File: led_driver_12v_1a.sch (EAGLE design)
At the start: 53 parts, among them Q1 BSZ0902NSI, Q2 BSZ0902NSI, Q3 BSZ0902NSI, Q4 BSZ0902NSI, Q5 BSZ0902NSI, Q6 SSM3K2615R

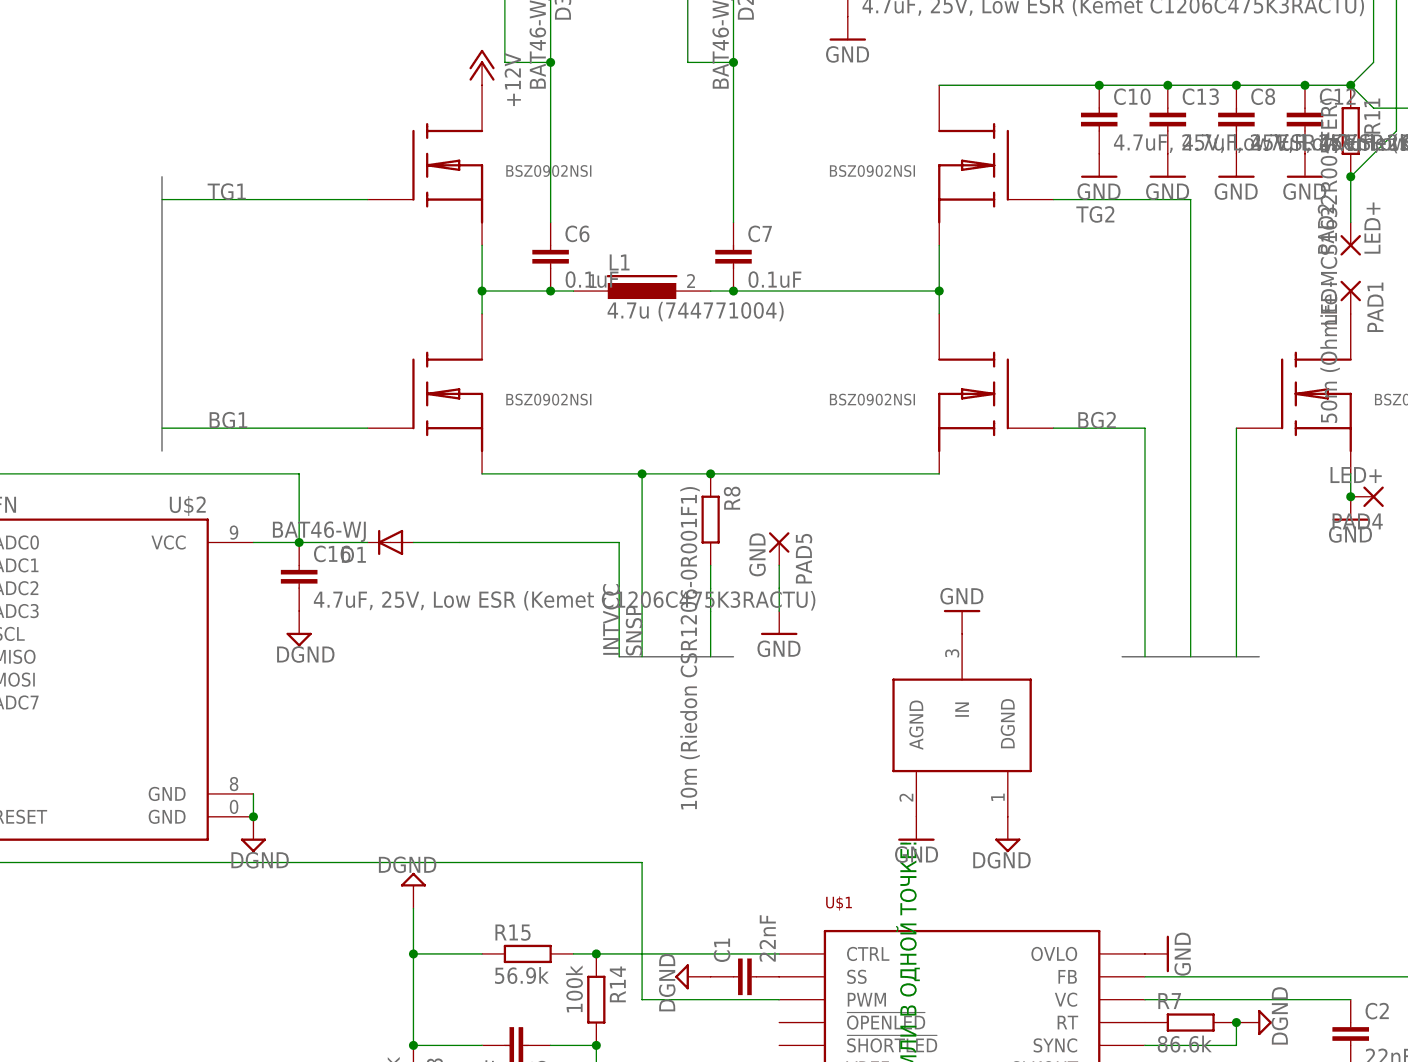
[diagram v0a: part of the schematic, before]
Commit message: routing complete. main tasks to do: add polys, optimize routes width, add some extra vias, make gerbers
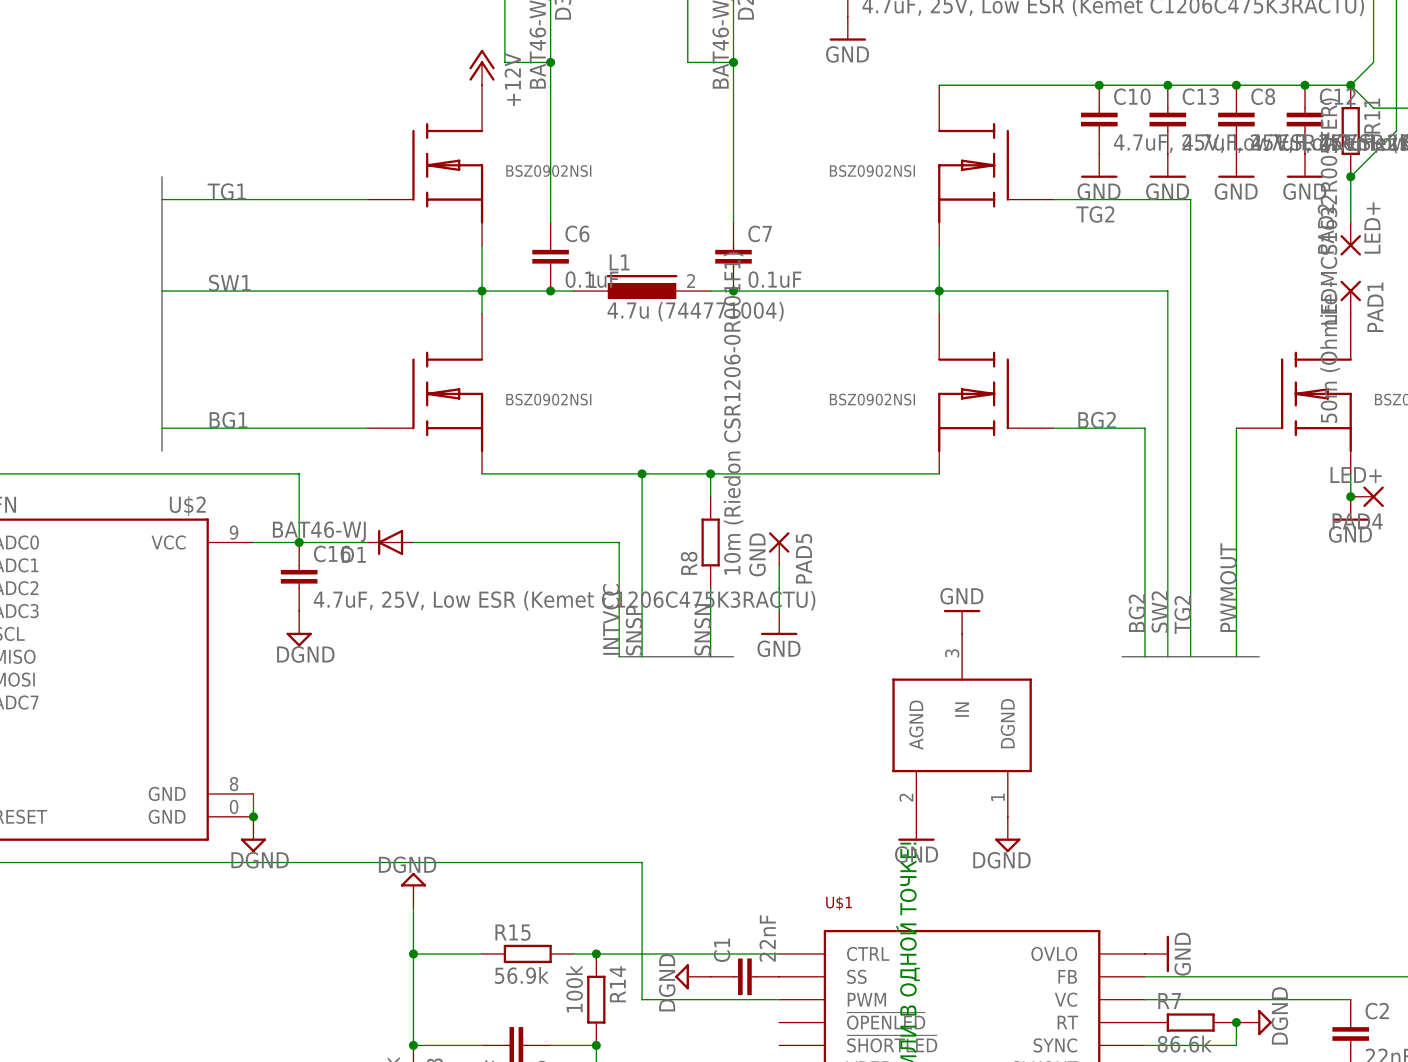
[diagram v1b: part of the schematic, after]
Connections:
- removed net N$10: C7.2, L1.2, Q3.D, Q4.S
- removed net N$8: C6.2, L1.1, Q1.S, Q2.D
- net SNSN: now also R8.1; no longer R8.2
- net SNSP: now also R8.2; no longer R8.1
- net SW1: now also C6.2, L1.1, Q1.S, Q2.D
- net SW2: now also C7.2, L1.2, Q3.D, Q4.S
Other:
- moved on the sheet: R8
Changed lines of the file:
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@@
 <clearance class="0" value="0.1524"/>
 </class>
-<class number="1" name="HI_PWR" width="0.3" drill="0.5">
+<class number="1" name="HI_PWR" width="0.3" drill="0.4">
 <clearance class="1" value="0.15"/>
 </class>
@@
 <instance part="Q3" gate="G$1" x="5.08" y="50.8" rot="MR0"/>
 <instance part="Q5" gate="G$1" x="45.72" y="50.8"/>
-<instance part="R8" gate="G$1" x="-22.86" y="38.1" rot="R270"/>
+<instance part="R8" gate="G$1" x="-22.86" y="35.56" rot="R90"/>
 <instance part="R11" gate="G$1" x="48.26" y="81.28" rot="R270"/>
 <instance part="D2" gate="G$1" x="-20.32" y="99.06" rot="R270"/>
@@
 <wire x1="25.4" y1="48.26" x2="25.4" y2="22.86" width="0.1524" layer="91"/>
 <label x="17.78" y="48.26" size="1.778" layer="95"/>
+<label x="25.4" y="25.4" size="1.778" layer="95" rot="R90"/>
 </segment>
 </net>
@@
 </segment>
 </net>
-<net name="SW2" class="0">
+<net name="SW2" class="1">
 <segment>
 <pinref part="U$1" gate="G$1" pin="SW2"/>
@@
 <label x="27.94" y="-53.34" size="1.778" layer="95"/>
 </segment>
-</net>
-<net name="SW1" class="0">
+<segment>
+<pinref part="L1" gate="G$1" pin="2"/>
+<pinref part="C7" gate="G$1" pin="2"/>
+<wire x1="-22.86" y1="63.5" x2="-20.32" y2="63.5" width="0.1524" layer="91"/>
+<pinref part="Q4" gate="G$1" pin="S"/>
+<wire x1="-20.32" y1="63.5" x2="2.54" y2="63.5" width="0.1524" layer="91"/>
+<wire x1="2.54" y1="63.5" x2="2.54" y2="68.58" width="0.1524" layer="91"/>
+<junction x="-20.32" y="63.5"/>
+<pinref part="Q3" gate="G$1" pin="D"/>
+<wire x1="2.54" y1="63.5" x2="2.54" y2="60.96" width="0.1524" layer="91"/>
+<junction x="2.54" y="63.5"/>
+<wire x1="27.94" y1="22.86" x2="27.94" y2="63.5" width="0.1524" layer="91"/>
+<wire x1="27.94" y1="63.5" x2="2.54" y2="63.5" width="0.1524" layer="91"/>
+<label x="27.94" y="25.4" size="1.778" layer="95" rot="R90"/>
+</segment>
+</net>
+<net name="SW1" class="1">
 <segment>
 <pinref part="U$1" gate="G$1" pin="SW1"/>
 <wire x1="-15.24" y1="-48.26" x2="-25.4" y2="-48.26" width="0.1524" layer="91"/>
 <label x="-22.86" y="-48.26" size="1.778" layer="95"/>
+</segment>
+<segment>
+<pinref part="Q1" gate="G$1" pin="S"/>
+<pinref part="Q2" gate="G$1" pin="D"/>
+<wire x1="-48.26" y1="68.58" x2="-48.26" y2="63.5" width="0.1524" layer="91"/>
+<pinref part="L1" gate="G$1" pin="1"/>
+<wire x1="-48.26" y1="63.5" x2="-48.26" y2="60.96" width="0.1524" layer="91"/>
+<wire x1="-38.1" y1="63.5" x2="-40.64" y2="63.5" width="0.1524" layer="91"/>
+<junction x="-48.26" y="63.5"/>
+<pinref part="C6" gate="G$1" pin="2"/>
+<wire x1="-40.64" y1="63.5" x2="-48.26" y2="63.5" width="0.1524" layer="91"/>
+<junction x="-40.64" y="63.5"/>
+<wire x1="-83.82" y1="63.5" x2="-48.26" y2="63.5" width="0.1524" layer="91"/>
+<label x="-78.74" y="63.5" size="1.778" layer="95"/>
 </segment>
 </net>
@@
 <wire x1="30.48" y1="73.66" x2="30.48" y2="22.86" width="0.1524" layer="91"/>
 <label x="17.78" y="71.12" size="1.778" layer="95"/>
+<label x="30.48" y="25.4" size="1.778" layer="95" rot="R90"/>
 </segment>
 </net>
@@
 </segment>
 </net>
-<net name="N$8" class="1">
-<segment>
-<pinref part="Q1" gate="G$1" pin="S"/>
-<pinref part="Q2" gate="G$1" pin="D"/>
-<wire x1="-48.26" y1="68.58" x2="-48.26" y2="63.5" width="0.1524" layer="91"/>
-<pinref part="L1" gate="G$1" pin="1"/>
-<wire x1="-48.26" y1="63.5" x2="-48.26" y2="60.96" width="0.1524" layer="91"/>
-<wire x1="-38.1" y1="63.5" x2="-40.64" y2="63.5" width="0.1524" layer="91"/>
-<junction x="-48.26" y="63.5"/>
-<pinref part="C6" gate="G$1" pin="2"/>
-<wire x1="-40.64" y1="63.5" x2="-48.26" y2="63.5" width="0.1524" layer="91"/>
-<junction x="-40.64" y="63.5"/>
-</segment>
-</net>
-<net name="N$10" class="1">
-<segment>
-<pinref part="L1" gate="G$1" pin="2"/>
-<pinref part="C7" gate="G$1" pin="2"/>
-<wire x1="-22.86" y1="63.5" x2="-20.32" y2="63.5" width="0.1524" layer="91"/>
-<pinref part="Q4" gate="G$1" pin="S"/>
-<wire x1="-20.32" y1="63.5" x2="2.54" y2="63.5" width="0.1524" layer="91"/>
-<wire x1="2.54" y1="63.5" x2="2.54" y2="68.58" width="0.1524" layer="91"/>
-<junction x="-20.32" y="63.5"/>
-<pinref part="Q3" gate="G$1" pin="D"/>
-<wire x1="2.54" y1="63.5" x2="2.54" y2="60.96" width="0.1524" layer="91"/>
-<junction x="2.54" y="63.5"/>
-</segment>
-</net>
 <net name="PWMOUT" class="1">
 <segment>
@@
 <pinref part="Q5" gate="G$1" pin="G"/>
 <wire x1="35.56" y1="48.26" x2="35.56" y2="22.86" width="0.1524" layer="91"/>
+<label x="35.56" y="25.4" size="1.778" layer="95" rot="R90"/>
 </segment>
 </net>
@@
 </segment>
 <segment>
-<pinref part="R8" gate="G$1" pin="2"/>
 <wire x1="-22.86" y1="22.86" x2="-22.86" y2="27.94" width="0.1524" layer="91"/>
-<wire x1="-22.86" y1="27.94" x2="-22.86" y2="30.48" width="0.1524" layer="91"/>
-<wire x1="-22.86" y1="30.48" x2="-22.86" y2="33.02" width="0.1524" layer="91"/>
+<pinref part="R8" gate="G$1" pin="1"/>
+<wire x1="-22.86" y1="30.48" x2="-22.86" y2="27.94" width="0.1524" layer="91"/>
+<label x="-22.86" y="22.86" size="1.778" layer="95" rot="R90"/>
 </segment>
 </net>
@@
 <segment>
 <pinref part="Q2" gate="G$1" pin="S"/>
+<wire x1="-48.26" y1="43.18" x2="-30.48" y2="43.18" width="0.1524" layer="91"/>
+<wire x1="-30.48" y1="22.86" x2="-30.48" y2="43.18" width="0.1524" layer="91"/>
+<label x="-30.48" y="22.86" size="1.778" layer="95" rot="R90"/>
 <pinref part="Q3" gate="G$1" pin="S"/>
-<wire x1="-48.26" y1="43.18" x2="-30.48" y2="43.18" width="0.1524" layer="91"/>
-<pinref part="R8" gate="G$1" pin="1"/>
 <wire x1="-30.48" y1="43.18" x2="-22.86" y2="43.18" width="0.1524" layer="91"/>
+<junction x="-30.48" y="43.18"/>
+<pinref part="R8" gate="G$1" pin="2"/>
 <wire x1="-22.86" y1="43.18" x2="2.54" y2="43.18" width="0.1524" layer="91"/>
+<wire x1="-22.86" y1="40.64" x2="-22.86" y2="43.18" width="0.1524" layer="91"/>
 <junction x="-22.86" y="43.18"/>
-<wire x1="-30.48" y1="22.86" x2="-30.48" y2="43.18" width="0.1524" layer="91"/>
-<junction x="-30.48" y="43.18"/>
-<label x="-30.48" y="22.86" size="1.778" layer="95" rot="R90"/>
-</segment>
-</net>
+</segment>
+</net>

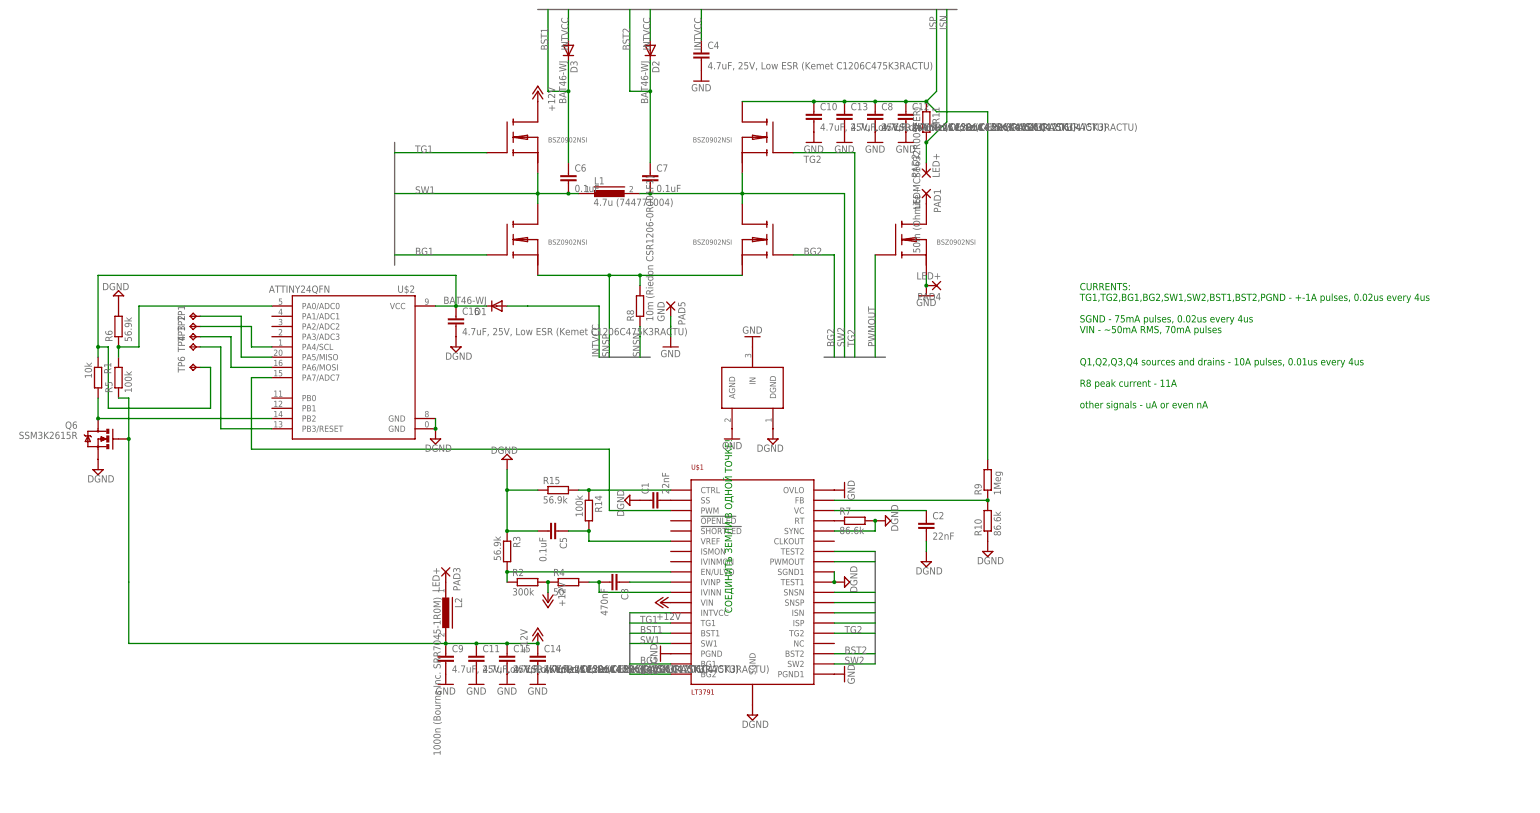
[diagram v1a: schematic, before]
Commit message: Added Gerbers and PartList
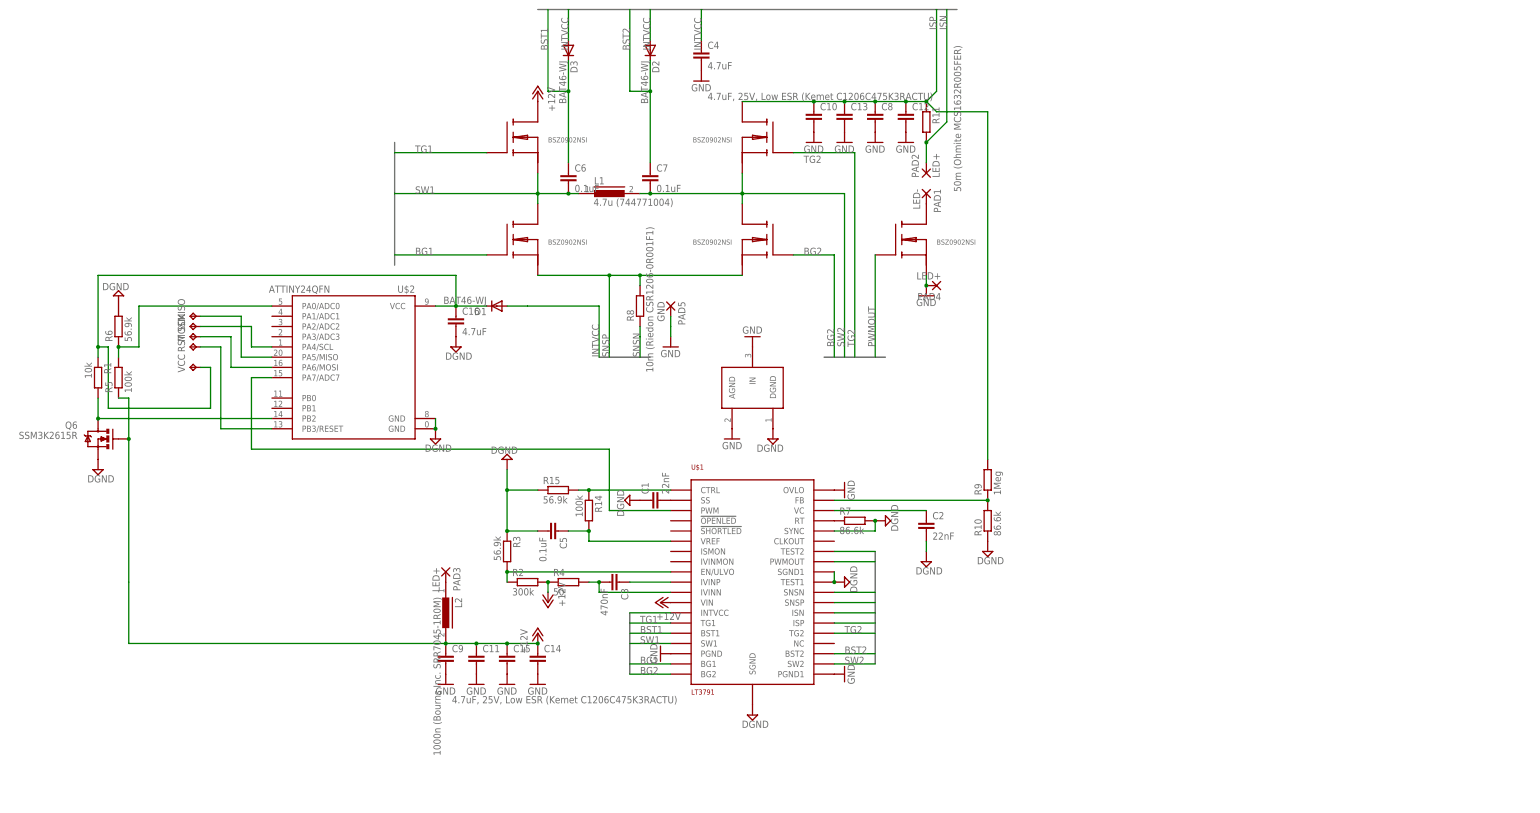
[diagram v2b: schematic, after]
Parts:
- C16, C4: value 4.7uF, 25V, Low ESR (Kemet C1206C475K3RACTU) -> 4.7uF
- renumbered TP1 to MISO, TP2 to SCK, TP3 to MOSI, TP4 to RST, TP6 to VCC
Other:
- note removed: "CURRENTS: TG1,TG2,BG1,BG2,SW1,SW2,BST1,BST2,PGND - +-1A pulses, 0.02us every 4us SGND - 75mA pulses, 0.02us every 4us VIN - ~50mA RMS, 70mA pulses Q1,Q2,Q3,Q4 sources and drains - 10A pulses, 0.01us every 4us R8 peak current - 11A other signals - uA or even nA"
- note removed: "СОЕДИНИТЬ ЗЕМЛИ В ОДНОЙ ТОЧКЕ!"
